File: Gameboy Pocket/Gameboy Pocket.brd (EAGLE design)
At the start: 70 x 57 mm, 44 parts, among them CN1 USB-SMD-NS, J3 battery, X3 16MHz

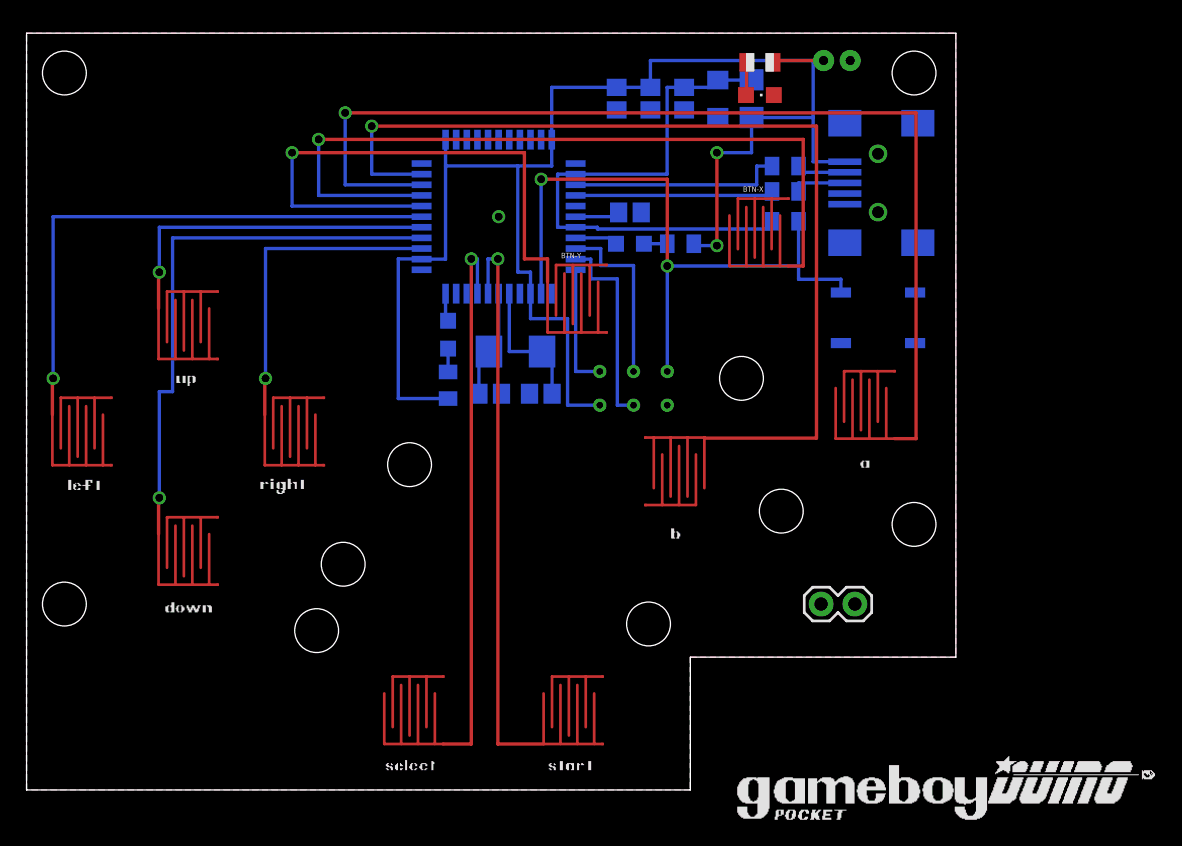
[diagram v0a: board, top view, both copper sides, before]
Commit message: Fri Mar 10 05:58:47 EST 2017
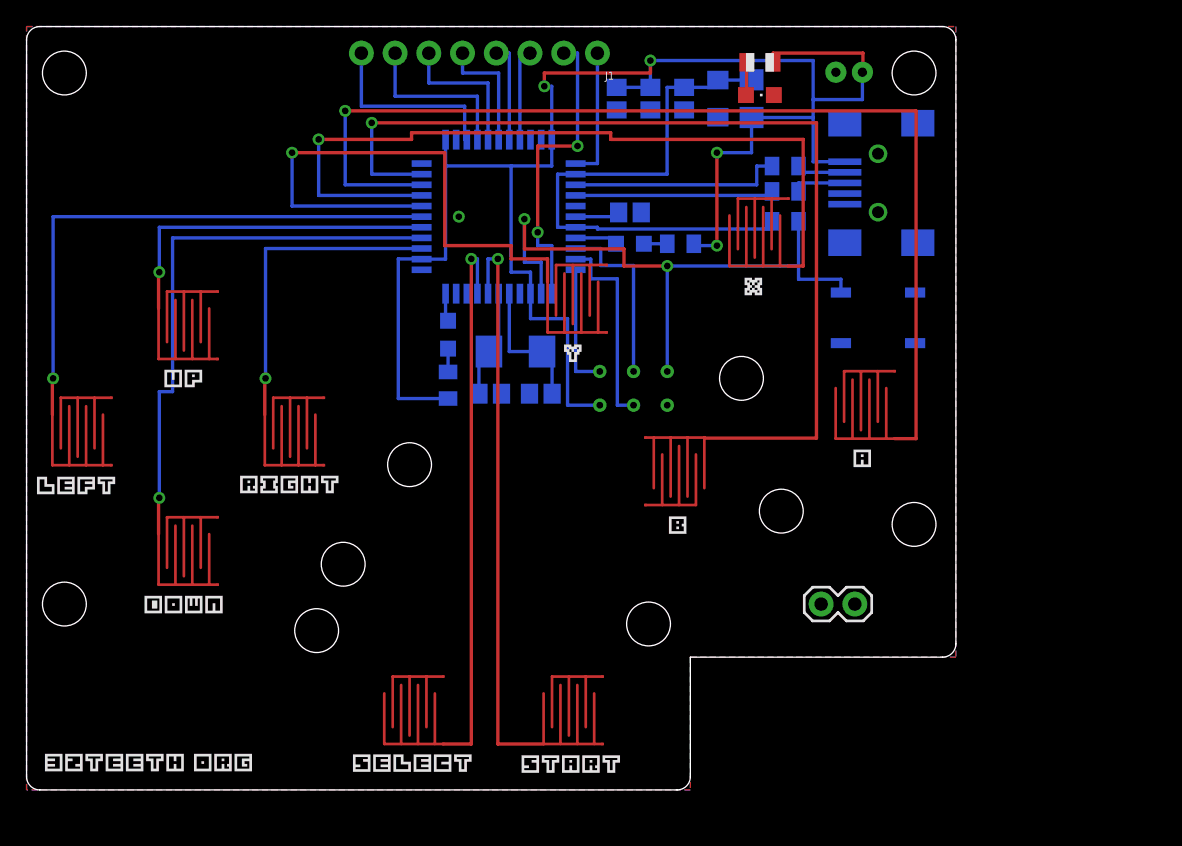
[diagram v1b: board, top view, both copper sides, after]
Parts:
- added J1: (no value), SparkFun-Connectors:1X08_NO_SILK
- moved J3 0.95 mm to (62.0, 54.6), turned to 0 degrees
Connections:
- new net HWB: U$2.33
- net A0: now also J1.8
- net A1: now also J1.7
- net A2: now also J1.6
- net A3: now also J1.5
- net A4: now also J1.4
- net A5: now also J1.3
- net D11: now also J1.2
- net D7: now also J1.1
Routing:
- net D11: track 0.00 -> 23.2 mm, vias 0 -> 2
- net VCC: track 120.2 -> 136.5 mm, vias 2 -> 4
- net A0: track 0.00 -> 14.5 mm
- net A1: track 0.00 -> 12.7 mm
- net A2: track 0.00 -> 11.0 mm
- net D7: track 0.00 -> 9.96 mm
- net A3: track 0.00 -> 9.24 mm
- net A4: track 0.00 -> 7.50 mm
- net A5: track 0.00 -> 7.28 mm
- net RST: track 51.0 -> 47.6 mm
- net D10/X: track 59.1 -> 60.1 mm
- net D13/B: track 72.9 -> 73.4 mm
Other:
- board size 70 x 57 mm -> 70 x 57.5 mm
- board text added: "A0 A1 A2 A3 A4 A5 D11 D7"

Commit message: Wed Mar 15 19:26:25 EDT 2017
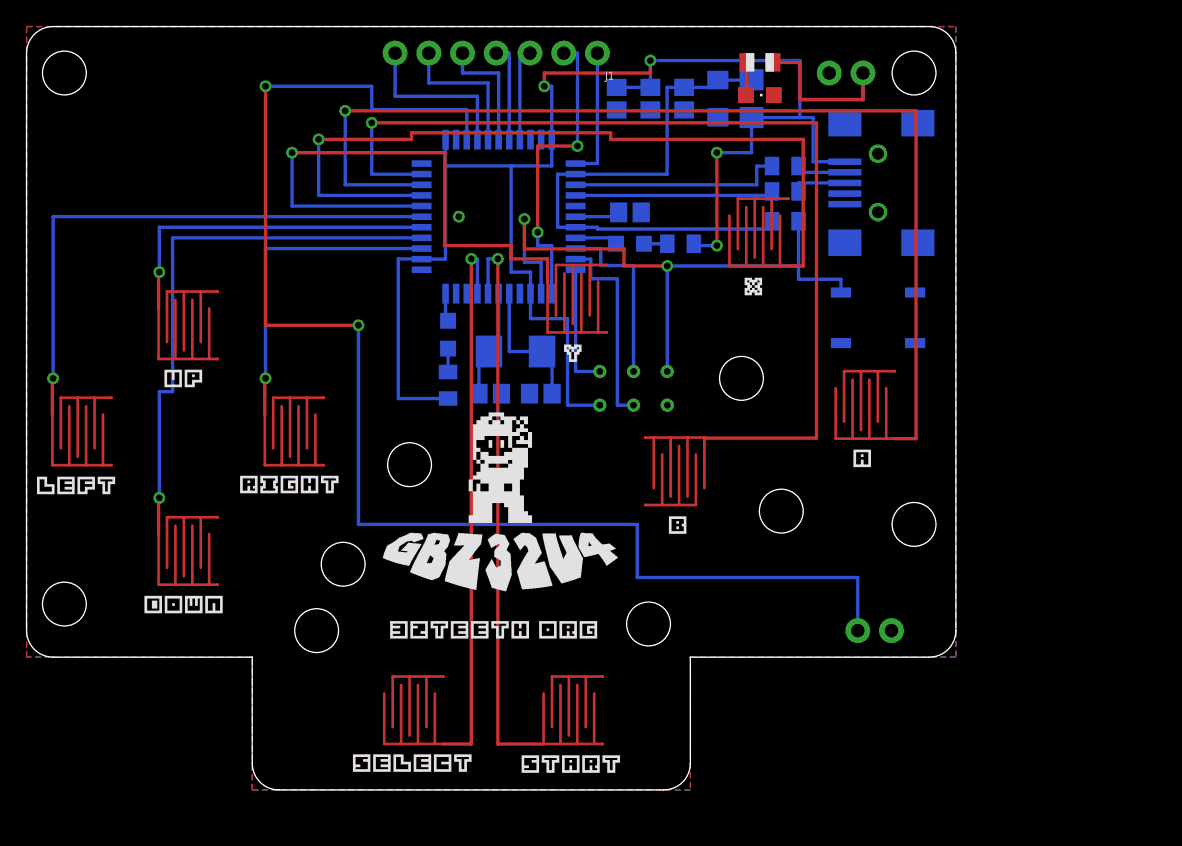
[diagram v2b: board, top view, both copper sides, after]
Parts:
- J1: device SparkFun-Connectors:1X08_NO_SILK -> SparkFun-Connectors:1X07_NO_SILK
- J3: device SparkFun-Connectors:JST-2-PTH-VERT -> SparkFun-Connectors:1X02_NO_SILK
- JP2: value (none) -> Speaker; device SparkFun-Connectors:1X02 -> SparkFun-Connectors:1X02_NO_SILK
- moved JP2 5.66 mm to (65.2, 12.0), turned to 180 degrees
- moved J3 1.21 mm to (63.0, 54.0)
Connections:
- removed net A0: J1.8, U$2.36
- removed net SPEAKER: JP2.2
- new net A0/SPEAKER: JP2.2, U$2.36
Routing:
- net A0/SPEAKER: track 0.00 -> 104.8 mm, vias 0 -> 2
- net A0: track 14.5 -> 0.00 mm
- net VCC: track 136.5 -> 139.1 mm
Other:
- outline, holes or cut-outs redrawn
- board text added: "/Users/eugeneandruszczenko/Desktop/logo.bmp"
- board text added: "D7 D11 A5 A4 A3 A2 A1"
- board text removed: "A0 A1 A2 A3 A4 A5 D11 D7"
